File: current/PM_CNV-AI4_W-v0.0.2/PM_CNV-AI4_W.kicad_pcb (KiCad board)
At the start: 2 copper layers, 79.8 x 99.8 mm, 74 parts, among them J1 AFA07-S10FCC-00, J2 AFA07-S10FCC-00, J4 15EDGRHC-THR-3.5-14P, J5 15EDGRHC-THR-3.5-14P, U1 AD7190BRUZ, U2 AD7190BRUZ, U3 CA-IS3761HW, U4 CA-IS3105W, U5 PM-LED8_v0.0.2

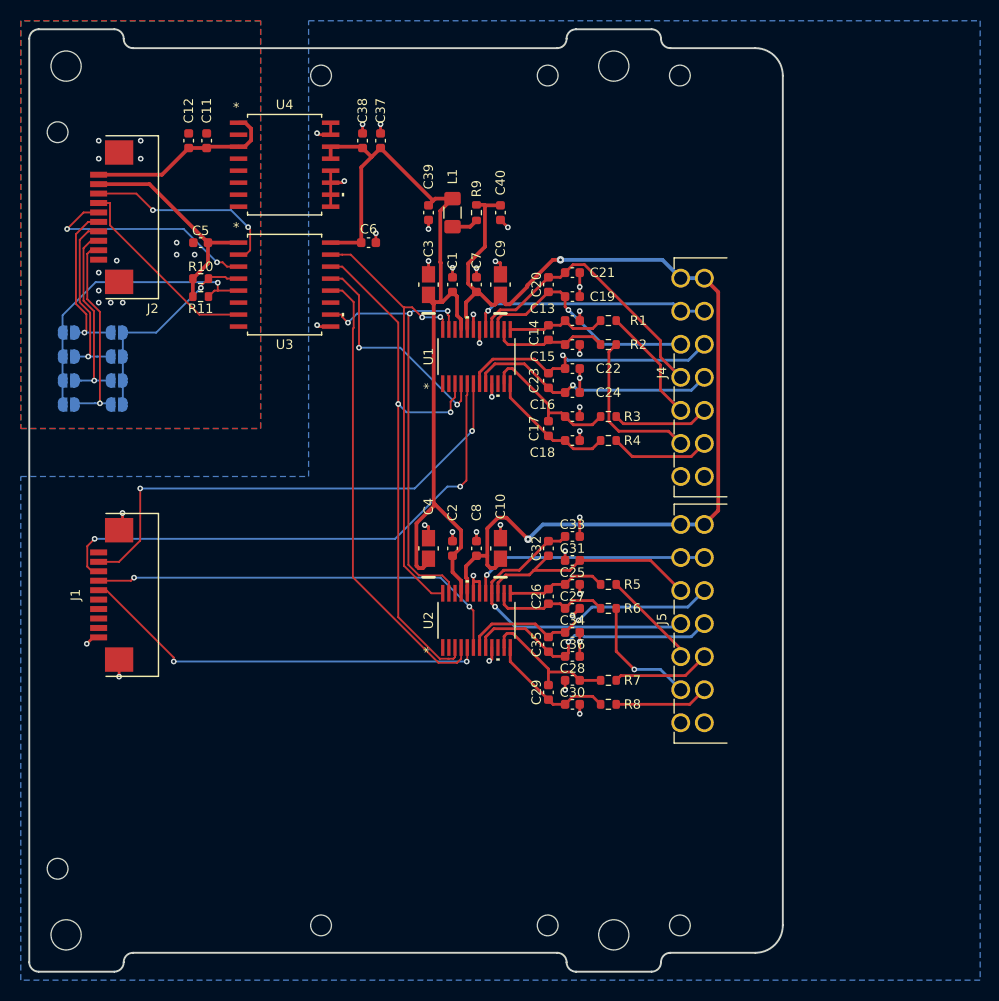
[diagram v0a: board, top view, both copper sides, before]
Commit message: PM_CNV-AI4_W-v0.0.2
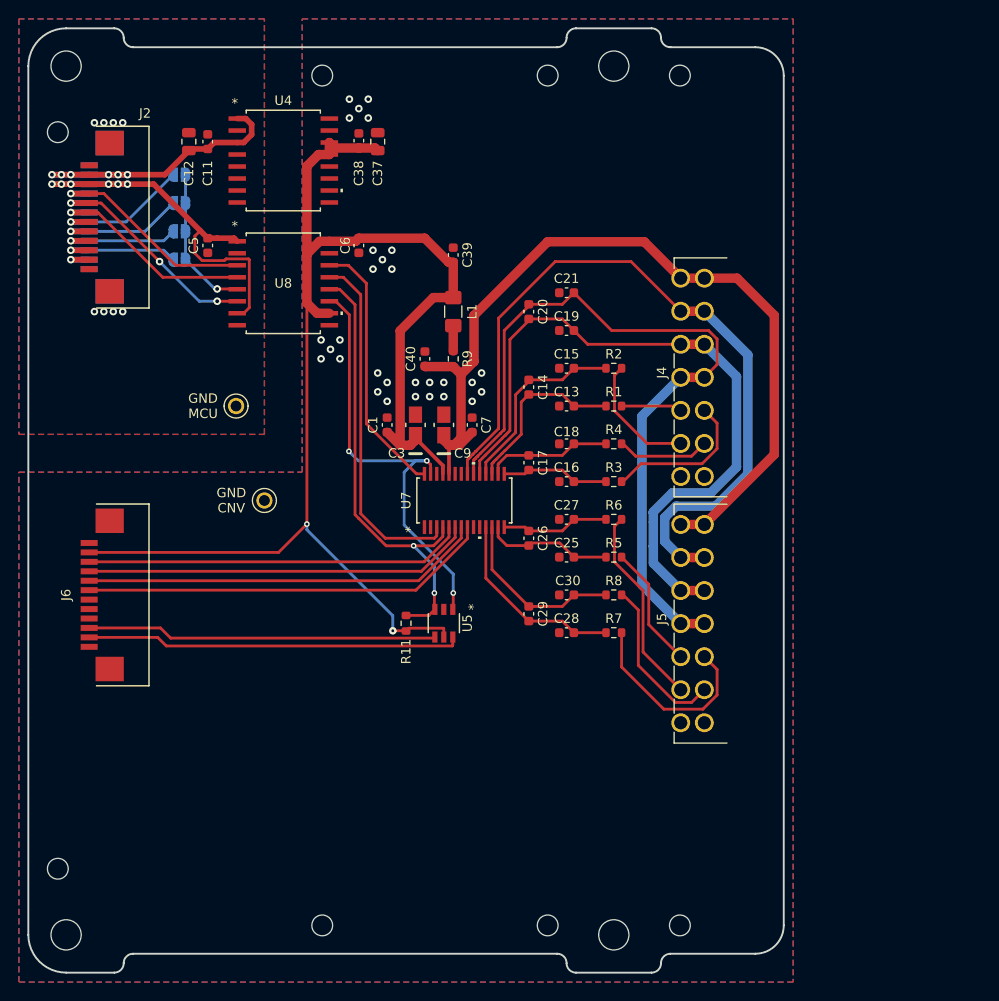
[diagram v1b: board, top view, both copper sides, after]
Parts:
- removed C10, C4: 10 uF, kicad_inventree_lib:TAJA_AVX-M
- removed C2, C8: 100nF, Capacitor_SMD:C_0603_1608Metric
- removed C22, C24, C31, C33, C34, C36: 10nF, Capacitor_SMD:C_0603_1608Metric
- removed C23, C32, C35: 1uF, Capacitor_SMD:C_0603_1608Metric
- removed J1: AFA07-S10FCC-00, kicad_inventree_lib:CONN10_AFA07-S10_JUS
- removed JP5, JP6, JP7, JP8: SolderJumper_2_Open, Jumper:SolderJumper-2_P1.3mm_Open_RoundedPad1.0x1.5mm
- removed R10: 10k, Resistor_SMD:R_0603_1608Metric
- removed U3: CA-IS3761HW, kicad_inventree_lib:SOIC16-WBW_CLG-M
- added J6: AFA07-S12FCC-00, kicad_inventree_lib:CONN10_AFA07-S12_JUS, F.Cu at (34.9, 110.3)
- added J7: AFA07-S12FCC-00, kicad_inventree_lib:CONN10_AFA07-S12_JUS, B.Cu at (34.9, 70.3)
- added SP1: ~, kicad_inventree_lib:PM_LED-xx-v0.0.1, F.Cu at (89.9, 100.3)
- added U7: AD7193BRUZ, kicad_inventree_lib:RU_28_ADI, F.Cu at (71.1, 100.3)
- added U8: CA-IS3741HW, kicad_inventree_lib:SOIC16-WBW_CLG-M, F.Cu at (51.9, 77.3)
- C12, C37: footprint Capacitor_SMD:C_0603_1608Metric -> Capacitor_SMD:C_0805_2012Metric
- J2: value AFA07-S10FCC-00 -> AFA07-S12FCC-00; footprint kicad_inventree_lib:CONN10_AFA07-S10_JUS -> kicad_inventree_lib:CONN10_AFA07-S12_JUS
- U1, U2: value AD7190BRUZ -> 5117; footprint kicad_inventree_lib:RU_24_ADI-M -> kicad_inventree_lib:5117
- U5: value PM-LED8_v0.0.2 -> SN74LVC2G14DBVR; footprint kicad_inventree_lib:PM-LED_v0.0.2 -> kicad_inventree_lib:DBV6-M
- U6: footprint kicad_inventree_lib:PM-ESP32C3_v0.0.4 -> kicad_inventree_lib:PM-ESP32C3_v0.0.5
- moved R11 40.9 mm to (64.9, 113.3), turned to 90 degrees
- moved U2 34.1 mm to (46.9, 90.3), turned to 0 degrees
- moved U1 27.1 mm to (49.9, 100.3), turned to 0 degrees
- moved U5 24.7 mm to (68.9, 113.3), turned to -90 degrees
- moved JP1 18.0 mm to (40.9, 65.8)
- moved JP2 17.6 mm to (40.9, 68.8)
- moved C40 17.4 mm to (66.9, 85.3), turned to 90 degrees
- moved JP3 17.1 mm to (40.9, 71.8)
- moved JP4 16.7 mm to (40.9, 74.8)
- moved C1 16.4 mm to (62.9, 92.3)
- moved C9 16.0 mm to (68.9, 92.3)
- moved R9 15.7 mm to (69.9, 85.3), turned to -90 degrees
- moved C3 14.9 mm to (65.9, 92.3)
- moved C7 14.9 mm to (71.9, 92.3)
- moved C30 11.6 mm to (81.9, 110.3), turned to 180 degrees
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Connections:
- net Net-(JP1-B) renamed /CS_MCU
- C1 pad 1: +5V_ISO -> +5V_CNV
- C1 pad 2: AGND -> GND_CNV
- C11 pad 1: +5V -> +5V_MCU
- C11 pad 2: GND -> GND_MCU
- C12 pad 1: +5V -> +5V_MCU
- C12 pad 2: GND -> GND_MCU
- C13 pad 1: AGND -> /AIN7
- C13 pad 2: /AD_0_AIN2 -> GND_CNV
- C14 pad 1: /AD_0_AIN2 -> /AIN7
- C14 pad 2: /AD_0_AIN3 -> /AIN8
- C15 pad 1: /AD_0_AIN3 -> /AIN8
- C15 pad 2: AGND -> GND_CNV
- C16 pad 1: AGND -> /AIN5
- C16 pad 2: /AD_0_AIN0 -> GND_CNV
- C17 pad 1: /AD_0_AIN0 -> /AIN5
- C17 pad 2: /AD_0_AIN1 -> /AIN6
- C18 pad 1: /AD_0_AIN1 -> /AIN6
- C18 pad 2: AGND -> GND_CNV
- C19 pad 1: AGND -> /SENSE+
- C19 pad 2: /0.SENSE+ -> GND_CNV
- C20 pad 1: /0.SENSE+ -> /SENSE+
- C20 pad 2: /0.SENSE- -> /SENSE-
- C21 pad 1: /0.SENSE- -> /SENSE-
- C21 pad 2: AGND -> GND_CNV
- C25 pad 1: AGND -> /AIN3
- C25 pad 2: /AD_1_AIN2 -> GND_CNV
- C26 pad 1: /AD_1_AIN2 -> /AIN3
- C26 pad 2: /AD_1_AIN3 -> /AIN4
- C27 pad 1: /AD_1_AIN3 -> /AIN4
- C27 pad 2: AGND -> GND_CNV
- C28 pad 1: AGND -> /AIN1
- C28 pad 2: /AD_1_AIN0 -> GND_CNV
- C29 pad 1: /AD_1_AIN0 -> /AIN1
- C29 pad 2: /AD_1_AIN1 -> /AIN2
- C3 pad 1: +5V_ISO -> +5V_CNV
- C3 pad 2: AGND -> GND_CNV
- C30 pad 1: /AD_1_AIN1 -> /AIN2
- C30 pad 2: AGND -> GND_CNV
- C37 pad 1: +5V_ISO -> +5V_CNV
- C37 pad 2: AGND -> GND_CNV
- C38 pad 1: +5V_ISO -> +5V_CNV
- C38 pad 2: AGND -> GND_CNV
- C39 pad 1: +5V_ISO -> +5V_CNV
- C39 pad 2: AGND -> GND_CNV
- C40 pad 1: AVDD -> +5V_CNV_FLT
- C40 pad 2: AGND -> GND_CNV
- C5 pad 1: +3.3V -> +3.3V_MCU
- C5 pad 2: GND -> GND_MCU
- C6 pad 1: +5V_ISO -> DGND
- C6 pad 2: AGND -> +5V_CNV
- C7 pad 1: AVDD -> +5V_CNV_FLT
- C7 pad 2: AGND -> GND_CNV
- C9 pad 1: AVDD -> +5V_CNV_FLT
- C9 pad 2: AGND -> GND_CNV
- J2 pad 1: GND -> GND_MCU
- J2 pad 10: +5V -> +3.3V_MCU
- J2 pad 11: GND -> +5V_MCU
- J2 pad 2: /CS3 -> /INT_MCU
- J2 pad 3: /CS2 -> /CS3_MCU
- J2 pad 4: /CS1 -> /CS2_MCU
- J2 pad 5: /CS0 -> /CS1_MCU
- J2 pad 6: /SCK -> /CS0_MCU
- J2 pad 7: /MISO -> /SCK_MCU
- J2 pad 8: /MOSI -> /MISO_MCU
- J2 pad 9: +3.3V -> /MOSI_MCU
- J4 pad 1: AGND -> GND_CNV
- J4 pad 11: /1.SENSE- -> /SENSE-
- J4 pad 12: /1.SENSE+ -> /SENSE+
- J4 pad 13: /0.EXC- -> /EXC-
- J4 pad 14: AVDD -> +5V_CNV_FLT
- J4 pad 4: /0.SENSE- -> /SENSE-
- J4 pad 5: /0.SENSE+ -> /SENSE+
- J4 pad 6: /0.EXC- -> /EXC-
- J4 pad 7: AVDD -> +5V_CNV_FLT
- J4 pad 8: AGND -> GND_CNV
- J5 pad 1: AGND -> GND_CNV
- J5 pad 11: /3.SENSE- -> /SENSE-
- J5 pad 12: /3.SENSE+ -> /SENSE+
- J5 pad 13: /2.EXC- -> /EXC-
- J5 pad 14: AVDD -> +5V_CNV_FLT
- J5 pad 4: /2.SENSE- -> /SENSE-
- J5 pad 5: /2.SENSE+ -> /SENSE+
- J5 pad 6: /2.EXC- -> /EXC-
- J5 pad 7: AVDD -> +5V_CNV_FLT
- J5 pad 8: AGND -> GND_CNV
- JP1 pad 1: /CS0 -> /CS0_MCU
- JP2 pad 1: /CS1 -> /CS1_MCU
- JP3 pad 1: /CS2 -> /CS2_MCU
- JP4 pad 1: /CS3 -> /CS3_MCU
- L1 pad 2: +5V_ISO -> +5V_CNV
- R1 pad 1: /AD_0_AIN2 -> /AIN7
- R11 pad 1: +3.3V -> +5V_CNV
- R11 pad 2: Net-(JP5-B) -> /CS_CNV
- R2 pad 1: /AD_0_AIN3 -> /AIN8
- R3 pad 1: /AD_0_AIN0 -> /AIN5
- R4 pad 1: /AD_0_AIN1 -> /AIN6
- R5 pad 1: /AD_1_AIN2 -> /AIN3
- R6 pad 1: /AD_1_AIN3 -> /AIN4
- R7 pad 1: /AD_1_AIN0 -> /AIN1
- R8 pad 1: /AD_1_AIN1 -> /AIN2
- R9 pad 2: AVDD -> +5V_CNV_FLT
- U1 pad 1: unconnected-(U1-MCLK1-Pad1) -> GND_CNV
- U2 pad 1: unconnected-(U2-MCLK1-Pad1) -> GND_MCU
- U4 pad 1: +5V -> +5V_MCU
- U4 pad 10: AGND -> GND_CNV
- U4 pad 11: AGND -> GND_CNV
- U4 pad 12: AGND -> GND_CNV
- U4 pad 13: +5V_ISO -> +5V_CNV
- U4 pad 14: +5V_ISO -> +5V_CNV
- U4 pad 15: AGND -> GND_CNV
- U4 pad 16: AGND -> GND_CNV
- U4 pad 2: GND -> GND_MCU
- U4 pad 3: +5V -> +5V_MCU
- U4 pad 4: GND -> GND_MCU
- U4 pad 5: GND -> GND_MCU
- U4 pad 6: GND -> GND_MCU
- U4 pad 7: GND -> GND_MCU
- U4 pad 8: GND -> GND_MCU
- U4 pad 9: AGND -> GND_CNV
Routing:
- net +5V_CNV: track 0.00 -> 145.9 mm, vias 0 -> 2
- net AVDD: track 109.8 -> 0.00 mm, vias 2 -> 0
- net +5V_ISO: track 93.2 -> 0.00 mm
- net +5V_CNV_FLT: track 0.00 -> 92.7 mm
- net /SENSE-: track 0.00 -> 82.0 mm
- net /EXC-: track 0.00 -> 81.6 mm
- net /SENSE+: track 0.00 -> 75.5 mm
- net /SCK_ISO: track 58.9 -> 0.00 mm, vias 2 -> 0
- net AGND: track 58.7 -> 0.00 mm, vias 37 -> 0
- net /LED1: track 56.9 -> 0.00 mm, vias 2 -> 0
- net /LED0: track 53.6 -> 0.00 mm, vias 2 -> 0
- net /CS1_ISO: track 48.7 -> 0.00 mm
- net /CS_CNV: track 0.00 -> 48.7 mm, vias 0 -> 2
- net /MOSI_ISO: track 48.5 -> 0.00 mm, vias 2 -> 0
- net /MISO_ISO: track 48.3 -> 0.00 mm, vias 3 -> 0
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- added copper zone on B.Cu, net GND_CNV
- added copper zone on F.Cu, net GND_CNV
- added copper zone on B.Cu, net GND_MCU
- added copper zone on F.Cu, net GND_MCU
- removed copper zone on B.Cu, net AGND
- removed copper zone on B.Cu, net GND
- removed copper zone on F.Cu, net GND
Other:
- board size 79.8 x 99.8 mm -> 80 x 100 mm
- board text added: "GND CNV"
- board text added: "GND MCU"
- board text added: "Shield"
- board text removed: "GND"
